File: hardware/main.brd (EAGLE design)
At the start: 99 x 99 mm, 37 parts, among them U1 TMS320F28069_PN_80, U10 TXB0101_DBV_6, U2 TXB0101_DBV_6, U3 TS3A5018_PW_16, U4 TS3A5018_PW_16, U5 SN74LVC4245A_DW_24, U7 Value, U8 Value, U9 SN74LVC4245A_DW_24

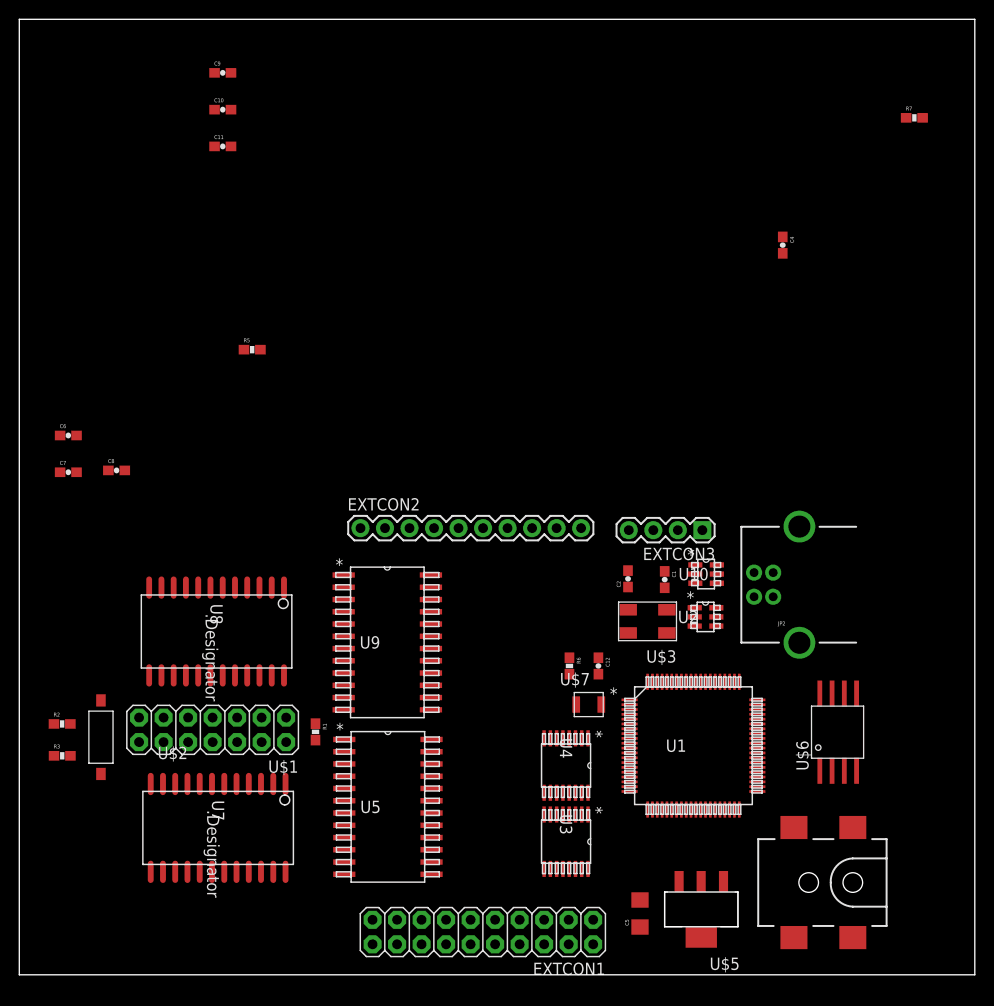
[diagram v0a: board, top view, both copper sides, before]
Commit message: Finished schematic, laid out board
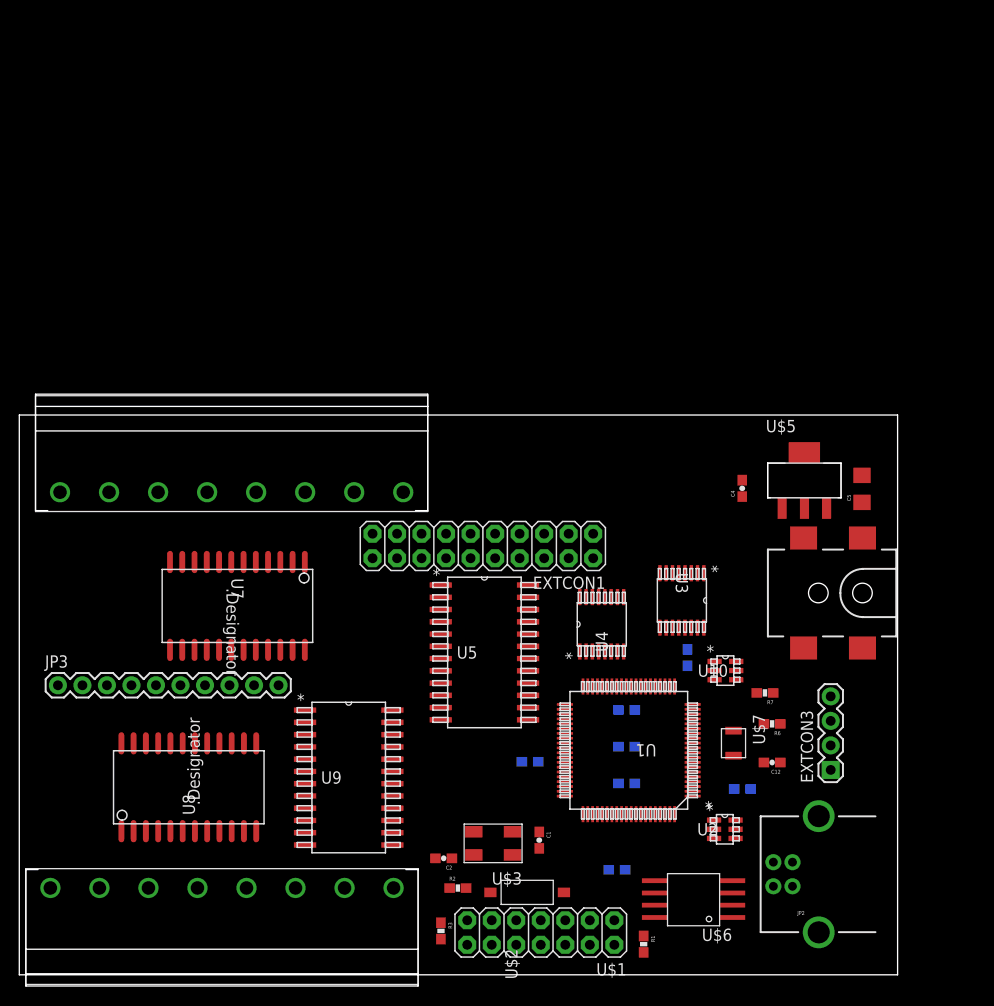
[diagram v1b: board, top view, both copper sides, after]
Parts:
- removed EXTCON2: M10SILK_FEMALE_PTH, SparkFun-Connectors:1X10
- added JP3: M10SILK_FEMALE_PTH, SparkFun-Connectors:1X10
- added U$4, U$8: 8PIN_SOCKET, ControllerCard:CONN-8PIN
- moved C10 78.1 mm to (62.9, 23.6), flipped to the bottom
- moved C11 78.1 mm to (62.9, 19.8), flipped to the bottom
- moved C9 78.1 mm to (62.9, 27.4), flipped to the bottom
- moved C8 72.8 mm to (74.9, 19.3), flipped to the bottom
- moved C6 72.5 mm to (61.9, 10.9), flipped to the bottom
- moved R7 61.6 mm to (77.3, 29.2), turned to 180 degrees
- moved C7 56.5 mm to (52.9, 22.1), flipped to the bottom
- moved R5 55.2 mm to (69.2, 32.9), flipped to the bottom, turned to 270 degrees
- moved C5 49.6 mm to (87.3, 50.4)
- moved U$2 47.0 mm to (52.6, 8.54), turned to 90 degrees
- moved U$5 45.7 mm to (81.3, 51.2), turned to 0 degrees
- moved R2 44.4 mm to (45.4, 8.99)
- moved R3 43.2 mm to (43.7, 4.55), turned to 270 degrees
- moved R1 40.5 mm to (64.7, 3.17)
- moved EXTCON1 40.0 mm to (48.0, 44.4)
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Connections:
- removed net IBUFIN1: U7.23
- removed net IBUFIN2: U7.22
- removed net IBUFIN3: U7.20
- removed net IBUFIN4: U7.19
- removed net IBUFIN5: U7.18
- removed net IBUFIN6: U7.17
- removed net IBUFIN7: U7.15
- removed net IBUFIN8: U7.14
- removed net OBUFIN1: U8.1
- removed net OBUFIN2: U8.3
- removed net OBUFIN3: U8.4
- removed net OBUFIN4: U8.6
- removed net OBUFIN5: U8.7
- removed net OBUFIN6: U8.9
- removed net OBUFIN7: U8.10
- removed net OBUFIN8: U8.12
- new net N$13: U$4.P$1, U8.1
- new net N$14: U$4.P$2, U8.3
- new net N$15: U$4.P$3, U8.4
- new net N$16: U$4.P$4, U8.6
- new net N$17: U$4.P$8, U8.12
- new net N$18: U$4.P$7, U8.10
- new net N$19: U$4.P$6, U8.9
- new net N$20: U$4.P$5, U8.7
- new net N$21: U$8.P$1, U7.23
- new net N$22: U$8.P$2, U7.22
- new net N$23: U$8.P$3, U7.20
- new net N$24: U$8.P$4, U7.19
- new net N$25: U$8.P$8, U7.14
- new net N$26: U$8.P$7, U7.15
- new net N$27: U$8.P$6, U7.17
- new net N$28: U$8.P$5, U7.18
- net !FLASHEN!: now also U1.78; no longer U1.45
- net !FLASHHOLD!: now also U1.80; no longer U1.46
- net !FLASHWP!: now also U1.79; no longer U1.43
- net 3.3V: no longer EXTCON2.1
- net 5V: now also JP3.10
- net BIN1: no longer EXTCON1.4
- net BIN2: no longer EXTCON1.6
- net BIN3: no longer EXTCON1.8
- net BIN4: no longer EXTCON1.10
- net BIN5: no longer EXTCON1.14
- net BIN6: no longer EXTCON1.16
- net BIN7: no longer EXTCON1.18
- net BIN8: no longer EXTCON1.20
- net GND: now also JP3.1; no longer EXTCON2.10
- net IBUFOUT1: now also EXTCON1.4
- net IBUFOUT2: now also EXTCON1.6
- net IBUFOUT3: now also EXTCON1.8
- net IBUFOUT4: now also EXTCON1.10
- net IBUFOUT5: now also EXTCON1.14
- net IBUFOUT6: now also EXTCON1.16
- net IBUFOUT7: now also EXTCON1.18
- net IBUFOUT8: now also EXTCON1.20
- net N$10: now also JP3.8
- net N$11: now also JP3.7
- net N$12: now also JP3.6
- net N$5: now also JP3.2
- net N$6: now also JP3.3
- net N$7: now also JP3.4
- net N$8: now also JP3.5
- net N$9: now also JP3.9
- net SPICLK: now also U1.76; no longer U1.41
- net SPISIMO: now also U1.77; no longer U1.44
- net SPISOMI: now also U1.75; no longer U1.42
- net UCIN1: now also U1.31; no longer U1.8
- net UCIN2: now also U1.32; no longer U1.31
- net UCIN3: now also U1.33; no longer U1.32
- net UCIN4: now also U1.34; no longer U1.33
- net UCIN5: now also U1.35; no longer U1.34
- net UCIN6: now also U1.39; no longer U1.35
- net UCIN7: now also U1.40; no longer U1.39
- net UCIN8: now also U1.41; no longer U1.40
- net UCOUT1: now also U1.42; no longer EXTCON2.2, U1.66
- net UCOUT2: now also U1.43; no longer EXTCON2.3, U1.67
- net UCOUT3: now also U1.44; no longer EXTCON2.4, U1.68
- net UCOUT4: now also U1.45; no longer EXTCON2.5, U1.69
- net UCOUT5: now also U1.46; no longer EXTCON2.6, U1.70
- net UCOUT6: now also U1.52; no longer EXTCON2.7, U1.75
- net UCOUT7: now also U1.53; no longer EXTCON2.8, U1.76
- net UCOUT8: now also U1.59; no longer EXTCON2.9, U1.77
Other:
- board size 99 x 99 mm -> 91 x 58 mm
